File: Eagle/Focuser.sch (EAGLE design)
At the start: 28 parts, among them IC1 L7805, IC2 L7805, Q1 IRF540, Q2 IRF540, Q3 IRF540

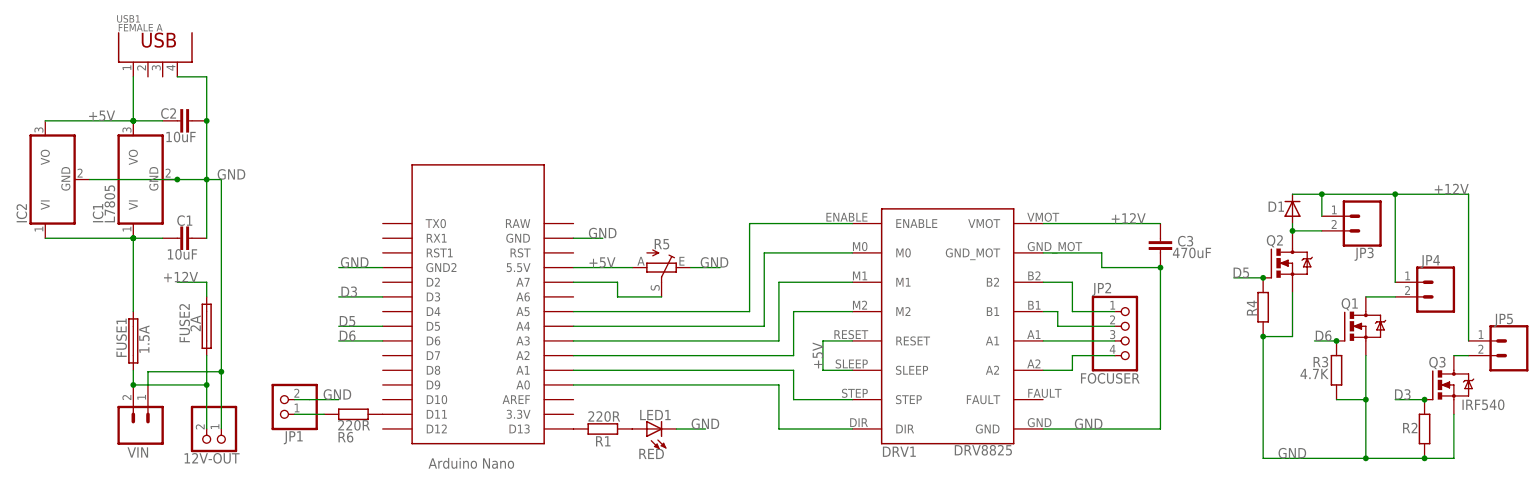
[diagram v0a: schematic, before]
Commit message: Circuit for commercial version
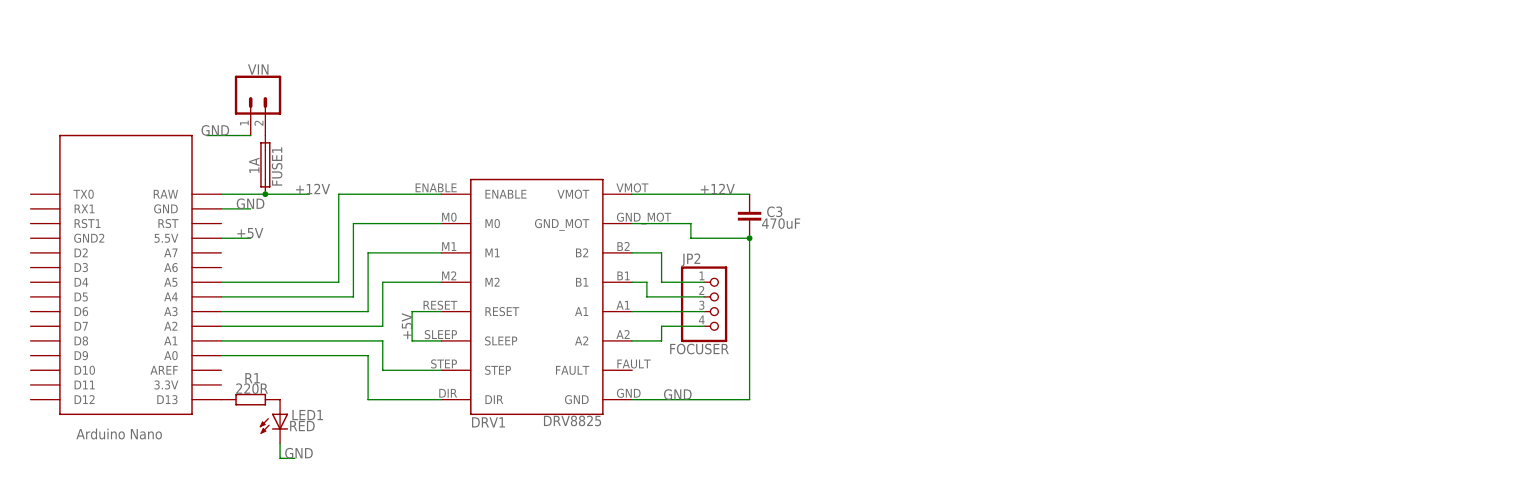
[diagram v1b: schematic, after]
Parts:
- removed 12V-OUT, JP1: (no value), pinhead:PINHD-1X2
- removed C1, C2: 10uF, rcl:C-EU025-024X044
- removed D1: (no value), diode:DIODE-D-2.5
- removed FUSE2: 2A, fuse:FUSEBLANK_5X20MM
- removed IC1, IC2: L7805, linear:786TV
- removed JP3, JP4, JP5: (no value), SparkFun-Connectors:CONN_025MM
- removed Q1, Q2, Q3: IRF540, transistor-power:IRF540
- removed R2, R3, R4: 4.7K, rcl:R-EU_0204/5
- removed R5: (no value), pot:TRIM_EU-B64Y
- removed R6: 220R, resistor:R-EU_0204/5
- removed USB1: FEMALE A, Seeed-Connector:DIP-USB-A-TYPE-FMAL(4+2P-2.0-90D)
- FUSE1: value 1.5A -> 1A
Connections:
- removed net D3: Q3.G, R2.2, U$1.D3
- removed net D5: Q2.G, R4.2, U$1.D5
- removed net D6: Q1.G, R3.2, U$1.D6
- removed net N$10: JP4.2, Q1.D
- removed net N$11: JP5.2, Q3.D
- removed net N$19: JP1.1, R6.1
- removed net N$2: R5.S, U$1.A7
- removed net N$3: R6.2, U$1.D11
- removed net N$4: C1.1, FUSE1.2, IC1.VI, IC2.VI
- removed net N$8: 12V-OUT.2, FUSE1.1, FUSE2.1, VIN.2
- removed net N$9: D1.A, JP3.2, Q2.D
- new net N$7: FUSE1.1, VIN.2
- net +12V: now also FUSE1.2, U$1.RAW; no longer D1.C, FUSE2.2, JP3.1, JP4.1, JP5.1
- net +5V: no longer C2.1, IC1.VO, IC2.VO, R5.A, USB1G$1.1
- net GND: no longer 12V-OUT.1, C1.2, C2.2, IC1.GND, IC2.GND, JP1.2, Q1.S, Q2.S, Q3.S, R2.1, R3.1, R4.1, R5.E, U$1.GND2, USB1G$1.4
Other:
- moved on the sheet: C3, DRV1, FUSE1, JP2, LED1, R1, VIN
